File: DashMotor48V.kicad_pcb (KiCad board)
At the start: 4 copper layers, 71.8 x 70.7 mm, 81 parts, among them CN3(OUT)1 XT30(2+2)PB-M.G.B, CN3(OUT)2 XT30(2+2)PB-M.G.B, J1 BM07B-SRSS-TB, J2 BM07B-SRSS-TB, Q1 FDMS039N08B, Q2 FDMS039N08B, Q3 FDMS039N08B, Q4 FDMS039N08B, Q5 FDMS039N08B, Q6 FDMS039N08B, U1 TPS629203DRLR, U2 TPS629203DRLR, U3 DRV8353SRTAR, U4 STM32F446RCT6, U5 MA732GQ-Z, U6 MCP2542FD-E/MF, Y1 CSTNE8M00G550000R0

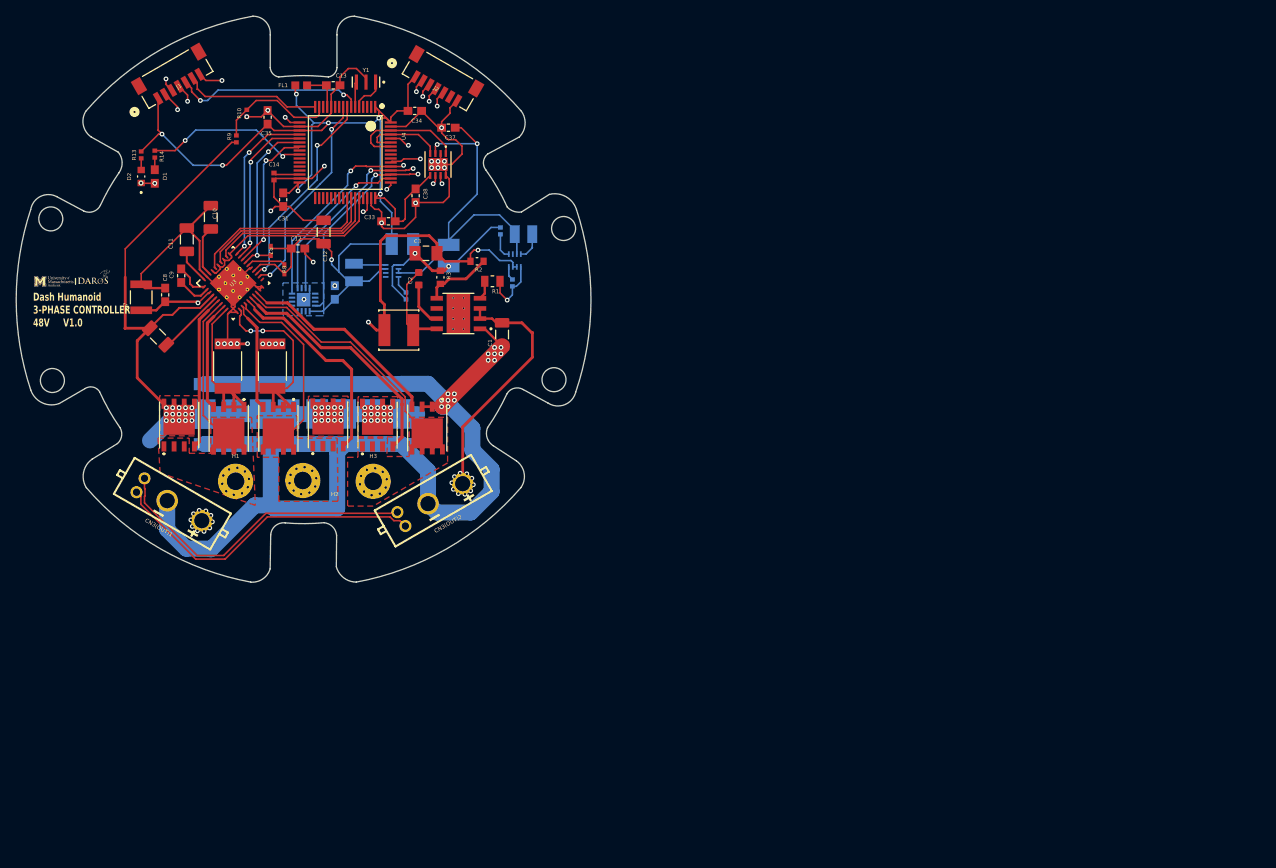
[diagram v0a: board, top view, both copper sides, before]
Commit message: will start 2nd version
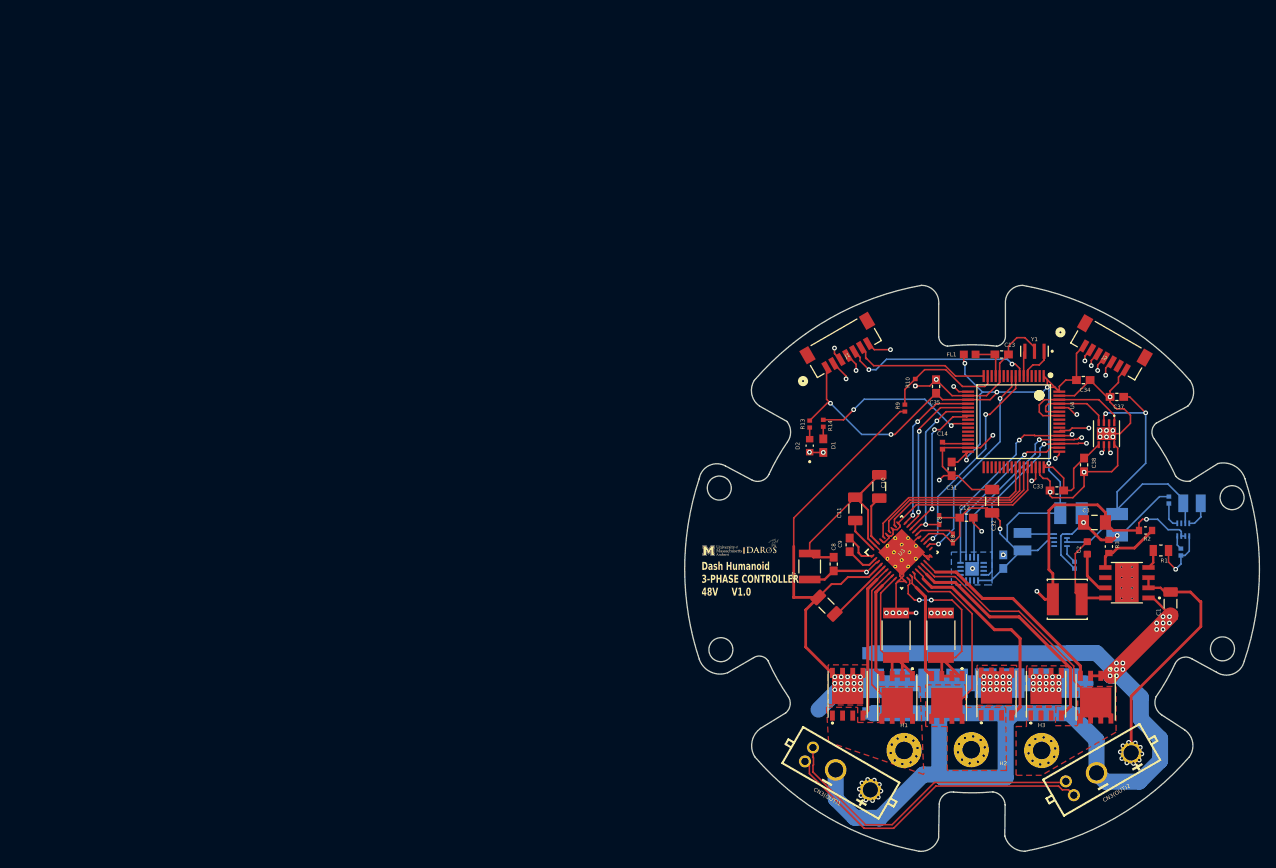
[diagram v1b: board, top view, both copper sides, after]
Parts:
- moved C1 90.1 mm to (174.8, 104.4)
- moved C2 90.1 mm to (164.4, 97.4)
- moved C26 90.1 mm to (137.6, 111.9)
- moved C27 90.1 mm to (141.1, 111.9)
- moved C28 90.1 mm to (144.6, 111.9)
- moved C29 90.1 mm to (148.1, 111.9)
- moved C36 90.1 mm to (153.9, 99.1)
- moved H2 90.1 mm to (149.9, 122.6)
- moved C10 90.1 mm to (138.4, 89.7)
- moved C11 90.1 mm to (135.4, 92.5)
- moved C19 90.1 mm to (151.7, 111.9)
- moved C20 90.1 mm to (155.2, 111.9)
- moved C21 90.1 mm to (158.7, 111.9)
- moved C22 90.1 mm to (148.1, 116.7)
- moved C23 90.1 mm to (144.6, 116.7)
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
